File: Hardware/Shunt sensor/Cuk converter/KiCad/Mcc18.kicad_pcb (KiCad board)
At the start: 2 copper layers, 199.1 x 107.2 mm, 61 parts, among them Q1 IRFP4321PbF, U1 INA240, U2 DRIVER_(INEP), U3 LM7812_TO220, U4 Signals_MCC, U5 ZCS, U6 INA211

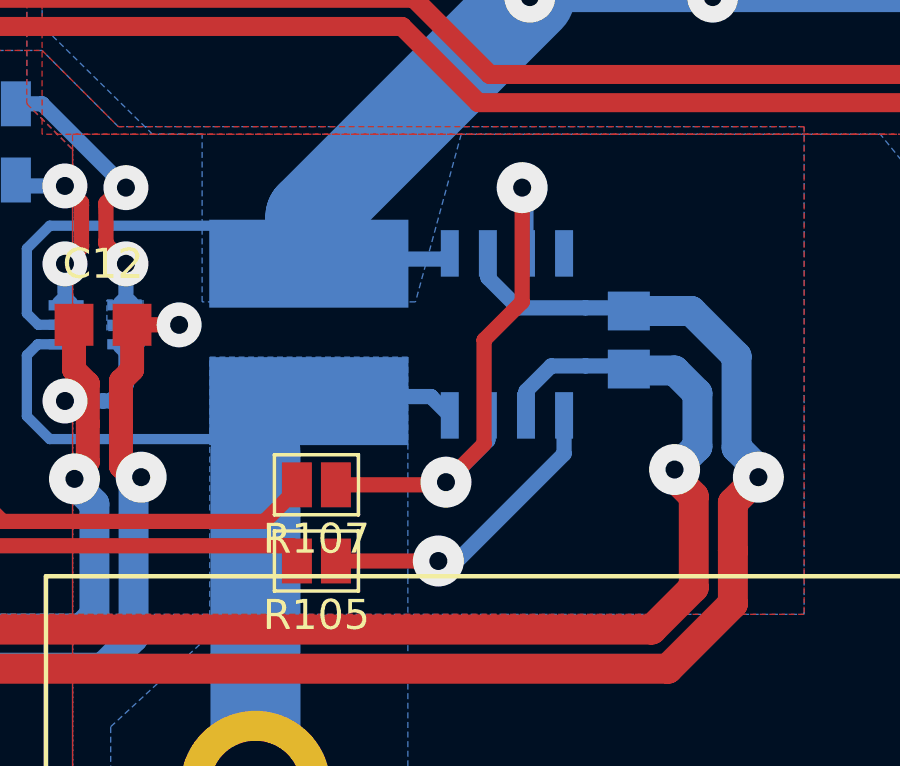
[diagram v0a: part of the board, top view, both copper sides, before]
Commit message: fixed clearance
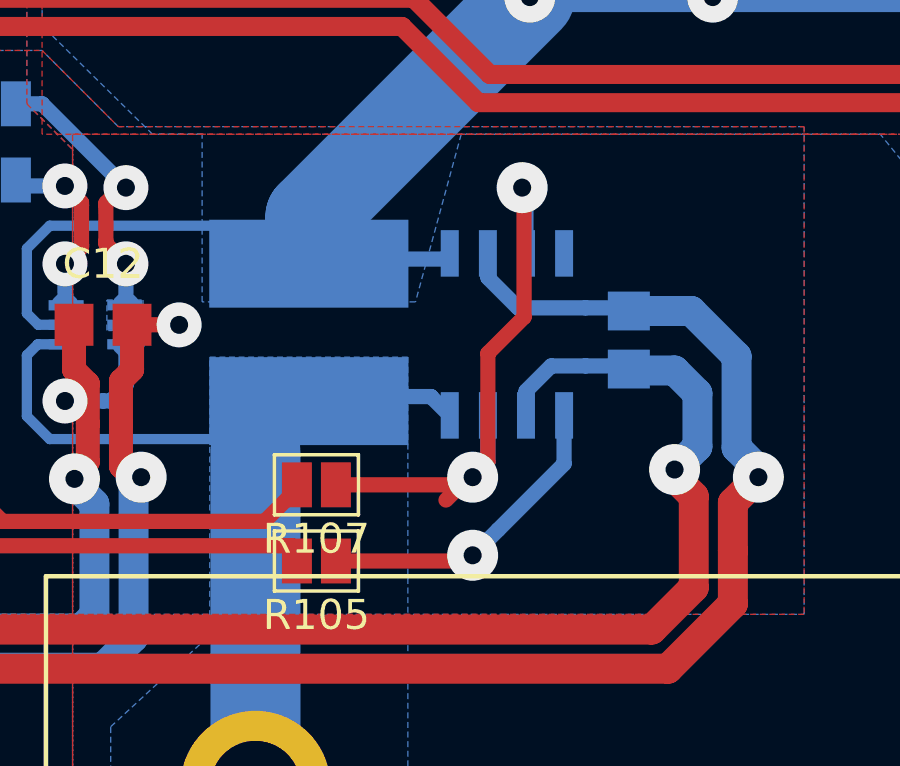
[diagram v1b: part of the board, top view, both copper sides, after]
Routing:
- net GNDA: track 135.8 -> 136.4 mm
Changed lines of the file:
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@@
     (thickness 1.6)
     (drawings 8)
-    (tracks 655)
+    (tracks 658)
     (zones 0)
     (modules 61)
@@
     (user_trace_width 9)
     (trace_clearance 0.3048)
-    (zone_clearance 0.3048)
+    (zone_clearance 1.27)
     (zone_45_only no)
     (trace_min 0.3429)
@@
   (segment (start 133.223 54.00804) (end 133.223 51.943) (width 0.508) (layer B.Cu) (net 25))
   (segment (start 133.223 51.943) (end 133.096 51.816) (width 0.508) (layer B.Cu) (net 25))
-  (via (at 130.556 61.633997) (size 1.7) (drill 0.6) (layers F.Cu B.Cu) (net 25))
-  (segment (start 130.556 62.23) (end 130.556 61.633997) (width 0.508) (layer F.Cu) (net 25))
-  (segment (start 131.953 60.236997) (end 131.953 59.40804) (width 0.508) (layer B.Cu) (net 25))
-  (segment (start 130.556 61.633997) (end 131.953 60.236997) (width 0.508) (layer B.Cu) (net 25))
-  (segment (start 131.826 60.363997) (end 130.556 61.633997) (width 0.508) (layer F.Cu) (net 25))
-  (segment (start 131.826 56.896) (end 131.826 60.363997) (width 0.508) (layer F.Cu) (net 25))
-  (segment (start 133.096 51.816) (end 133.096 55.626) (width 0.508) (layer F.Cu) (net 25))
-  (segment (start 133.096 55.626) (end 131.826 56.896) (width 0.508) (layer F.Cu) (net 25))
-  (segment (start 130.467997 61.722) (end 130.556 61.633997) (width 0.508) (layer F.Cu) (net 25))
-  (segment (start 126.888 61.722) (end 130.467997 61.722) (width 0.508) (layer F.Cu) (net 25))
   (via (at 98.806 50.292) (size 1.8) (drill 0.7) (layers F.Cu B.Cu) (net 25))
   (segment (start 101.1405 50.292) (end 99.314 50.292) (width 0.508) (layer B.Cu) (net 25))
@@
   (segment (start 116.22 49.022) (end 117.094 49.022) (width 0.508) (layer B.Cu) (net 25))
   (segment (start 117.094 49.022) (end 119.888 51.816) (width 0.508) (layer B.Cu) (net 25))
+  (via (at 131.445006 61.468) (size 1.7) (drill 0.6) (layers F.Cu B.Cu) (net 25))
+  (segment (start 131.953 60.960006) (end 131.445006 61.468) (width 0.508) (layer B.Cu) (net 25))
+  (segment (start 130.556 62.23) (end 131.318 61.468) (width 0.508) (layer F.Cu) (net 25))
+  (segment (start 131.953 59.40804) (end 131.953 60.960006) (width 0.508) (layer B.Cu) (net 25))
+  (segment (start 131.191006 61.722) (end 131.445006 61.468) (width 0.508) (layer F.Cu) (net 25))
+  (segment (start 126.888 61.722) (end 131.191006 61.722) (width 0.508) (layer F.Cu) (net 25))
+  (segment (start 131.318 61.468) (end 131.445006 61.468) (width 0.508) (layer F.Cu) (net 25))
+  (segment (start 131.953 60.960006) (end 131.445006 61.468) (width 0.508) (layer F.Cu) (net 25))
+  (segment (start 131.953 57.3405) (end 131.953 60.960006) (width 0.508) (layer F.Cu) (net 25))
+  (segment (start 133.1595 56.134) (end 131.953 57.3405) (width 0.508) (layer F.Cu) (net 25))
+  (segment (start 133.096 51.816) (end 133.1595 51.8795) (width 0.508) (layer F.Cu) (net 25))
+  (segment (start 133.1595 51.8795) (end 133.1595 56.134) (width 0.508) (layer F.Cu) (net 25))
   (segment (start 119.94515 57.037999) (end 120.3579 57.037999) (width 0.3429) (layer B.Cu) (net 26))
   (segment (start 118.1585 56.388) (end 118.1585 56.4365) (width 0.3429) (layer F.Cu) (net 26))
@@
   (segment (start 114.3 62.738) (end 115.316 63.754) (width 0.508) (layer F.Cu) (net 60))
   (segment (start 115.316 63.754) (end 125.42521 63.754) (width 0.508) (layer F.Cu) (net 60))
-  (via (at 130.302 64.262) (size 1.7) (drill 0.6) (layers F.Cu B.Cu) (net 61))
-  (segment (start 126.888 64.262) (end 130.302 64.262) (width 0.508) (layer F.Cu) (net 61))
-  (segment (start 134.493 60.69104) (end 134.493 59.40804) (width 0.508) (layer B.Cu) (net 61))
-  (segment (start 130.302 64.262) (end 130.92204 64.262) (width 0.508) (layer B.Cu) (net 61))
-  (segment (start 130.92204 64.262) (end 134.493 60.69104) (width 0.508) (layer B.Cu) (net 61))
+  (via (at 131.445 64.0715) (size 1.7) (drill 0.6) (layers F.Cu B.Cu) (net 61))
+  (segment (start 126.888 64.262) (end 131.2545 64.262) (width 0.508) (layer F.Cu) (net 61))
+  (segment (start 131.2545 64.262) (end 131.445 64.0715) (width 0.508) (layer F.Cu) (net 61))
+  (segment (start 134.493 59.40804) (end 134.493 61.0235) (width 0.508) (layer B.Cu) (net 61))
+  (segment (start 134.493 61.0235) (end 132.294999 63.221501) (width 0.508) (layer B.Cu) (net 61))
+  (segment (start 132.294999 63.221501) (end 131.445 64.0715) (width 0.508) (layer B.Cu) (net 61))
   (via (at 117.856 54.356002) (size 1.5) (drill 0.6) (layers F.Cu B.Cu) (net 62))
   (segment (start 117.8941 54.394102) (end 117.856 54.356002) (width 0.3429) (layer B.Cu) (net 62))
@@
   )
   (zone (net 63) (net_name /Rs+) (layer B.Cu) (hatch full 0.508)
-    (priority 26)
-    (connect_pads yes (clearance 0.3048))
-    (min_thickness 0.254)
+    (priority 6)
+    (connect_pads yes (clearance 1.27))
+    (min_thickness 0.508)
     (fill yes (arc_segments 16) (thermal_gap 0.3048) (thermal_bridge_width 0.3048) (smoothing fillet) (radius 2))
     (polygon
@@
   )
   (zone (net 25) (net_name GNDA) (layer B.Cu) (hatch full 0.508)
-    (priority 25)
+    (priority 5)
     (connect_pads yes (clearance 0.3048))
     (min_thickness 0.508)
@@
   )
   (zone (net 25) (net_name GNDA) (layer F.Cu) (hatch full 0.508)
-    (priority 25)
+    (priority 5)
     (connect_pads yes (clearance 0.3048))
     (min_thickness 0.508)
@@
   )
   (zone (net 46) (net_name /-Vp) (layer B.Cu) (hatch edge 0.508)
-    (priority 3)
+    (priority 6)
     (connect_pads yes (clearance 1.27))
     (min_thickness 0.508)
-    (fill yes (arc_segments 16) (thermal_gap 0.508) (thermal_bridge_width 0.508) (smoothing fillet) (radius 4))
+    (fill yes (arc_segments 16) (thermal_gap 0.508) (thermal_bridge_width 0.508) (smoothing chamfer) (radius 3.81))
     (polygon
       (pts
@@
       )
     )
+  )
+  (zone (net 0) (net_name "") (layer B.Cu) (hatch full 0.508)
+    (connect_pads yes (clearance 0.3048))
+    (min_thickness 0.508)
+    (keepout (tracks allowed) (vias allowed) (copperpour not_allowed))
+    (fill (arc_segments 16) (thermal_gap 0.508) (thermal_bridge_width 0.508) (smoothing chamfer) (radius 2))
+    (polygon
+      (pts
+        (xy 129.4765 55.8165) (xy 129.4765 56.261) (xy 129.4765 57.2135) (xy 129.4765 57.404) (xy 129.4765 57.4675)
+        (xy 122.682 57.4675) (xy 122.682 57.15) (xy 122.682 56.3245) (xy 122.682 55.8165)
+      )
+    )
